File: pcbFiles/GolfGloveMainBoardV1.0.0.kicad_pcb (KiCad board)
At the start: 4 copper layers, 40 x 55.3 mm, 78 parts, among them J1 USB_C_Receptacle, J11 Conn_01x16_Male, J12 HOST_WAKE, J13 TP4, J14 Conn_01x02, J15 Conn_01x02, J16 Conn_01x02, J17 Conn_01x02, J2 Conn_01x06, J3 USB_C_Receptacle, J6 Screw_Terminal_01x02, J7 Conn_01x02, J8 Conn_01x02, J9 Conn_01x02, SW1 SW_SPDT, SW2 SW_Push, U1 MCP73831T-2ACI/OT, U2 XC6119N16A7R-G, U3 LSM9DS1TR, U4 CYW20719B1KUMLG, U5 LSM9DS1TR, U7 TPS63001DRCT, Y1 Crystal, Y2 Crystal_GND23

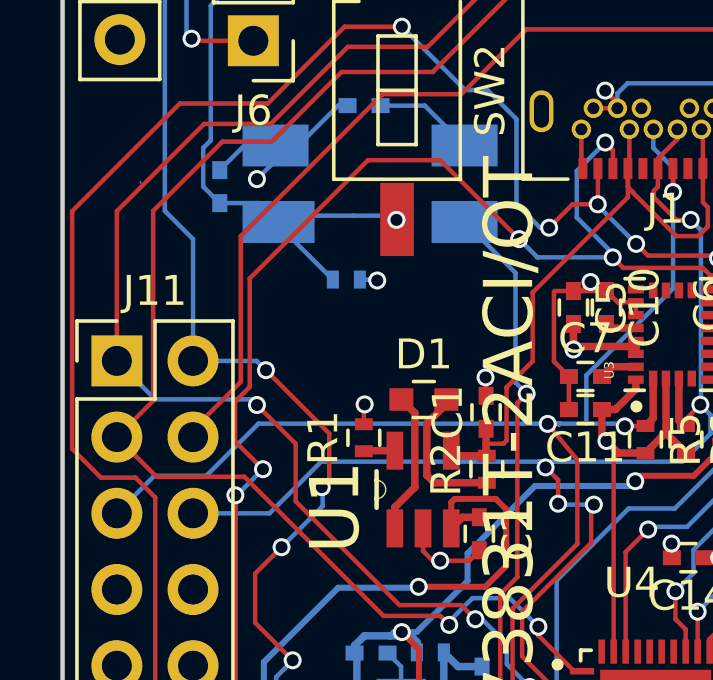
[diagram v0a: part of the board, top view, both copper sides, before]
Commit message: Update Fills and Outlines
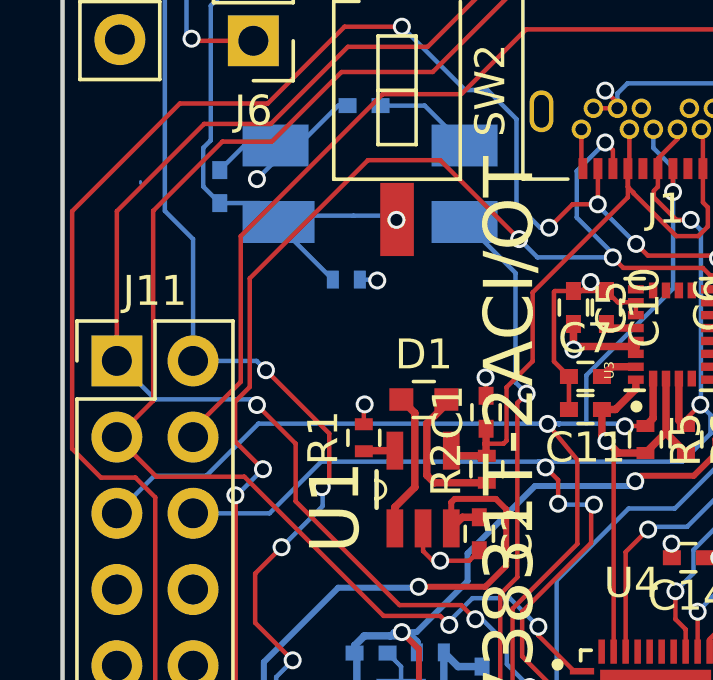
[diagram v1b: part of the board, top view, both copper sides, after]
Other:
- net class Default: via_dia 0.6 -> 0.5; via_drill 0.4 -> 0.34
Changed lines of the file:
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@@
-(kicad_pcb (version 4) (host pcbnew 4.0.7)
+(kicad_pcb (version 20171130) (host pcbnew "(5.0.2)-1")
   (general
-    (links 216)
-    (no_connects 3)
-    (area 102.504999 106.804999 142.645001 162.275001)
     (thickness 1.6)
     (drawings 27)
@@
   (layers
     (0 F.Cu signal)
-    (1 In1.Cu signal hide)
-    (2 In2.Cu signal hide)
+    (1 In1.Cu signal)
+    (2 In2.Cu signal)
     (31 B.Cu signal)
     (32 B.Adhes user)
@@
     (segment_width 0.2)
     (edge_width 0.15)
-    (via_size 0.6)
-    (via_drill 0.4)
+    (via_size 0.5)
+    (via_drill 0.34)
     (via_min_size 0.4)
     (via_min_drill 0.3)
@@
     (pad_drill 0.762)
     (pad_to_mask_clearance 0.2)
+    (solder_mask_min_width 0.25)
     (aux_axis_origin 0 0)
     (visible_elements 7FFEFFFF)
@@
       (layerselection 0x00030_80000001)
       (usegerberextensions false)
+      (usegerberattributes false)
+      (usegerberadvancedattributes false)
+      (creategerberjobfile false)
       (excludeedgelayer true)
       (linewidth 0.100000)
@@
       (hpglpennumber 1)
       (hpglpenspeed 20)
-      (hpglpendiameter 15)
-      (hpglpenoverlay 2)
+      (hpglpendiameter 15.000000)
       (psnegative false)
       (psa4output false)
@@
     (clearance 0.15)
     (trace_width 0.15)
-    (via_dia 0.6)
-    (via_drill 0.4)
+    (via_dia 0.5)
+    (via_drill 0.34)
     (uvia_dia 0.3)
     (uvia_drill 0.1)
@@
     (fp_line (start 5.8 2.4) (end 5.8 -2.4) (layer F.CrtYd) (width 0.05))
     (fp_line (start 5.8 -2.4) (end -5.8 -2.4) (layer F.CrtYd) (width 0.05))
-    (fp_text user %R (at 2.575 0 360) (layer F.Fab)
+    (fp_text user %R (at 2.575 0) (layer F.Fab)
       (effects (font (size 0.6 0.6) (thickness 0.15)))
     )
@@
     (fp_line (start 0.3048 -1.5494) (end -0.3048 -1.5494) (layer F.SilkS) (width 0.1524))
     (fp_line (start -0.3048 -1.5494) (end -0.6096 -1.5494) (layer F.SilkS) (width 0.1524))
-    (fp_arc (start 0 -1.5494) (end -0.3048 -1.5494) (angle -180) (layer F.SilkS) (width 0))
+    (fp_arc (start 0 -1.5494) (end -0.3048 -1.5494) (angle -180) (layer F.SilkS) (width 0.1))
     (fp_line (start -0.8636 1.5494) (end 0.8636 1.5494) (layer Dwgs.User) (width 0.1524))
     (fp_line (start 0.8636 1.5494) (end 0.8636 1.1938) (layer Dwgs.User) (width 0.1524))
@@
     (fp_line (start 1.4986 -0.7112) (end 1.4986 -1.1938) (layer Dwgs.User) (width 0.1524))
     (fp_line (start 1.4986 -1.1938) (end 0.8636 -1.1938) (layer Dwgs.User) (width 0.1524))
-    (fp_arc (start 0 -1.5494) (end -0.3048 -1.5494) (angle -180) (layer Dwgs.User) (width 0))
+    (fp_arc (start 0 -1.5494) (end -0.3048 -1.5494) (angle -180) (layer Dwgs.User) (width 0.1))
     (pad 1 smd rect (at -1.2954 -0.9398 90) (size 1.27 0.5588) (layers F.Cu F.Paste F.Mask)
       (net 25 "Net-(D1-Pad1)"))
@@
       (effects (font (size 0.812819 0.812819) (thickness 0.05)) (justify mirror))
     )
-    (fp_line (start 0.15 0) (end 3.45 0) (layer Eco2.User) (width 0))
-    (fp_line (start 3.75 0) (end 7.05 0) (layer Eco2.User) (width 0))
-    (fp_line (start 7.2 0.15) (end 7.2 1.2) (layer Eco2.User) (width 0))
-    (fp_line (start 7.2 1.45) (end 7.2 3.75) (layer Eco2.User) (width 0))
-    (fp_line (start 7.2 4) (end 7.2 5.05) (layer Eco2.User) (width 0))
-    (fp_line (start 7.05 5.2) (end 3.75 5.2) (layer Eco2.User) (width 0))
-    (fp_line (start 3.45 5.2) (end 0.15 5.2) (layer Eco2.User) (width 0))
-    (fp_line (start 0 5.05) (end 0 4) (layer Eco2.User) (width 0))
-    (fp_line (start 0 3.75) (end 0 1.45) (layer Eco2.User) (width 0))
-    (fp_line (start 0 1.2) (end 0 0.15) (layer Eco2.User) (width 0))
-    (fp_line (start 11.25 2.61) (end 11.25 2.67) (layer B.Cu) (width 0))
-    (fp_arc (start 0 3.875) (end 0 3.75) (angle 180) (layer Eco2.User) (width 0))
-    (fp_arc (start 0 1.325) (end 0 1.2) (angle 180) (layer Eco2.User) (width 0))
-    (fp_arc (start 0.0375 0.0375) (end 0.15 0) (angle 126.8) (layer Eco2.User) (width 0))
-    (fp_arc (start 3.6 0) (end 3.75 0) (angle 180) (layer Eco2.User) (width 0))
-    (fp_arc (start 3.6 5.2) (end 3.45 5.2) (angle 180) (layer Eco2.User) (width 0))
-    (fp_arc (start 0.0375 5.1625) (end 0 5.05) (angle 126.8) (layer Eco2.User) (width 0))
-    (fp_arc (start 7.2 3.875) (end 7.2 4) (angle 180) (layer Eco2.User) (width 0))
-    (fp_arc (start 7.2 1.325) (end 7.2 1.45) (angle 180) (layer Eco2.User) (width 0))
-    (fp_arc (start 7.1625 5.1625) (end 7.05 5.2) (angle 126.8) (layer Eco2.User) (width 0))
-    (fp_arc (start 7.1625 0.0375) (end 7.2 0.15) (angle 126.8) (layer Eco2.User) (width 0))
+    (fp_line (start 0.15 0) (end 3.45 0) (layer Eco2.User) (width 0.1))
+    (fp_line (start 3.75 0) (end 7.05 0) (layer Eco2.User) (width 0.1))
+    (fp_line (start 7.2 0.15) (end 7.2 1.2) (layer Eco2.User) (width 0.1))
+    (fp_line (start 7.2 1.45) (end 7.2 3.75) (layer Eco2.User) (width 0.1))
+    (fp_line (start 7.2 4) (end 7.2 5.05) (layer Eco2.User) (width 0.1))
+    (fp_line (start 7.05 5.2) (end 3.75 5.2) (layer Eco2.User) (width 0.1))
+    (fp_line (start 3.45 5.2) (end 0.15 5.2) (layer Eco2.User) (width 0.1))
+    (fp_line (start 0 5.05) (end 0 4) (layer Eco2.User) (width 0.1))
+    (fp_line (start 0 3.75) (end 0 1.45) (layer Eco2.User) (width 0.1))
+    (fp_line (start 0 1.2) (end 0 0.15) (layer Eco2.User) (width 0.1))
+    (fp_line (start 11.25 2.61) (end 11.25 2.67) (layer B.Cu) (width 0.1))
+    (fp_arc (start 0 3.875) (end 0 3.75) (angle 180) (layer Eco2.User) (width 0.1))
+    (fp_arc (start 0 1.325) (end 0 1.2) (angle 180) (layer Eco2.User) (width 0.1))
+    (fp_arc (start 0.0375 0.0375) (end 0.15 0) (angle 126.8) (layer Eco2.User) (width 0.1))
+    (fp_arc (start 3.6 0) (end 3.75 0) (angle 180) (layer Eco2.User) (width 0.1))
+    (fp_arc (start 3.6 5.2) (end 3.45 5.2) (angle 180) (layer Eco2.User) (width 0.1))
+    (fp_arc (start 0.0375 5.1625) (end 0 5.05) (angle 126.8) (layer Eco2.User) (width 0.1))
+    (fp_arc (start 7.2 3.875) (end 7.2 4) (angle 180) (layer Eco2.User) (width 0.1))
+    (fp_arc (start 7.2 1.325) (end 7.2 1.45) (angle 180) (layer Eco2.User) (width 0.1))
+    (fp_arc (start 7.1625 5.1625) (end 7.05 5.2) (angle 126.8) (layer Eco2.User) (width 0.1))
+    (fp_arc (start 7.1625 0.0375) (end 7.2 0.15) (angle 126.8) (layer Eco2.User) (width 0.1))
     (pad 2 smd rect (at 0.45 3.87 180) (size 2.2 1.4) (layers B.Cu B.Paste B.Mask)
       (net 5 "Net-(C3-Pad1)"))
@@
     (fp_line (start -1.5748 -1.5748) (end 1.5748 -1.5748) (layer B.SilkS) (width 0.1524))
     (fp_line (start 1.5748 1.5748) (end -1.5748 1.5748) (layer B.SilkS) (width 0.1524))
-    (fp_line (start -1.5748 -1.5748) (end 1.5748 -1.5748) (layer Dwgs.User) (width 0))
-    (fp_line (start 1.5748 -1.5748) (end 1.5748 1.5748) (layer Dwgs.User) (width 0))
-    (fp_line (start 1.5748 1.5748) (end 0.3048 1.5748) (layer Dwgs.User) (width 0))
-    (fp_line (start 0.3048 1.5748) (end -0.3048 1.5748) (layer Dwgs.User) (width 0))
-    (fp_line (start -0.3048 1.5748) (end -1.5748 1.5748) (layer Dwgs.User) (width 0))
-    (fp_line (start -1.5748 1.5748) (end -1.5748 -1.5748) (layer Dwgs.User) (width 0))
-    (fp_arc (start 0 1.5748) (end -0.3048 1.5748) (angle 180) (layer Dwgs.User) (width 0))
+    (fp_line (start -1.5748 -1.5748) (end 1.5748 -1.5748) (layer Dwgs.User) (width 0.1))
+    (fp_line (start 1.5748 -1.5748) (end 1.5748 1.5748) (layer Dwgs.User) (width 0.1))
+    (fp_line (start 1.5748 1.5748) (end 0.3048 1.5748) (layer Dwgs.User) (width 0.1))
+    (fp_line (start 0.3048 1.5748) (end -0.3048 1.5748) (layer Dwgs.User) (width 0.1))
+    (fp_line (start -0.3048 1.5748) (end -1.5748 1.5748) (layer Dwgs.User) (width 0.1))
+    (fp_line (start -1.5748 1.5748) (end -1.5748 -1.5748) (layer Dwgs.User) (width 0.1))
+    (fp_arc (start 0 1.5748) (end -0.3048 1.5748) (angle 180) (layer Dwgs.User) (width 0.1))
     (pad 1 smd rect (at -1.4732 0.9906) (size 0.8128 0.3048) (layers B.Cu B.Paste B.Mask)
       (net 7 3.3v))
@@
     (polygon
       (pts
-        (xy 142.57 125.65) (xy 142.57 160.65) (xy 102.58 160.65) (xy 102.58 125.66)
+        (xy 142.57 125.65) (xy 142.55 162.25) (xy 102.6 162.2) (xy 102.58 125.66)
       )
     )
@@
     (polygon
       (pts
-        (xy 142.57 125.65) (xy 142.57 160.65) (xy 102.57 160.65) (xy 102.57 125.65)
+        (xy 142.57 125.65) (xy 142.5 162.25) (xy 102.55 162.25) (xy 102.57 125.65)
       )
     )
